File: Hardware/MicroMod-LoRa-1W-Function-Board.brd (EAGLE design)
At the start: 67.5 x 38 mm, 48 parts, among them J11 MICROMOD_STANDARD, Q3 20V/4.2A/52mΩ/1.4W, Q4 600mA/40V, Q5 20V/4.2A/52mΩ/1.4W, Q6 600mA/40V, U1 EEPROM, U4 E19-915M30S

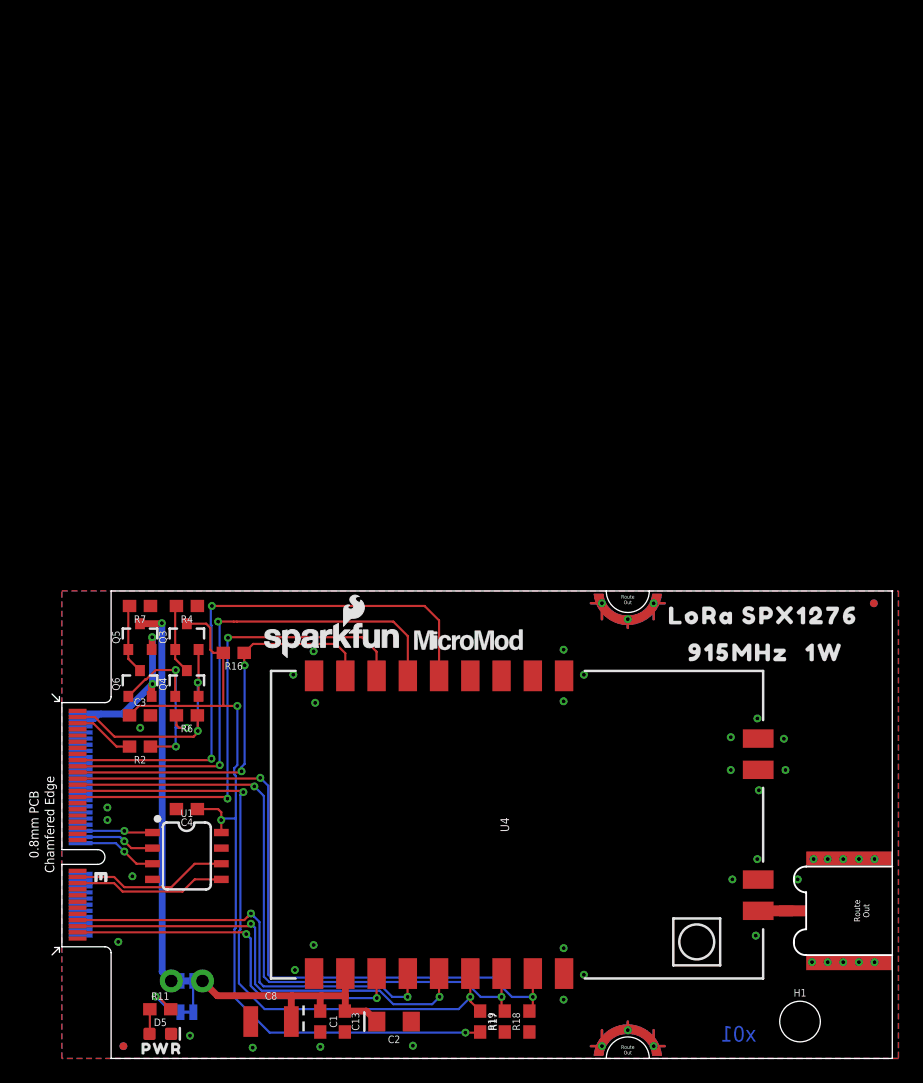
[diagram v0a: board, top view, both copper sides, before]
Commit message: Adding panel files
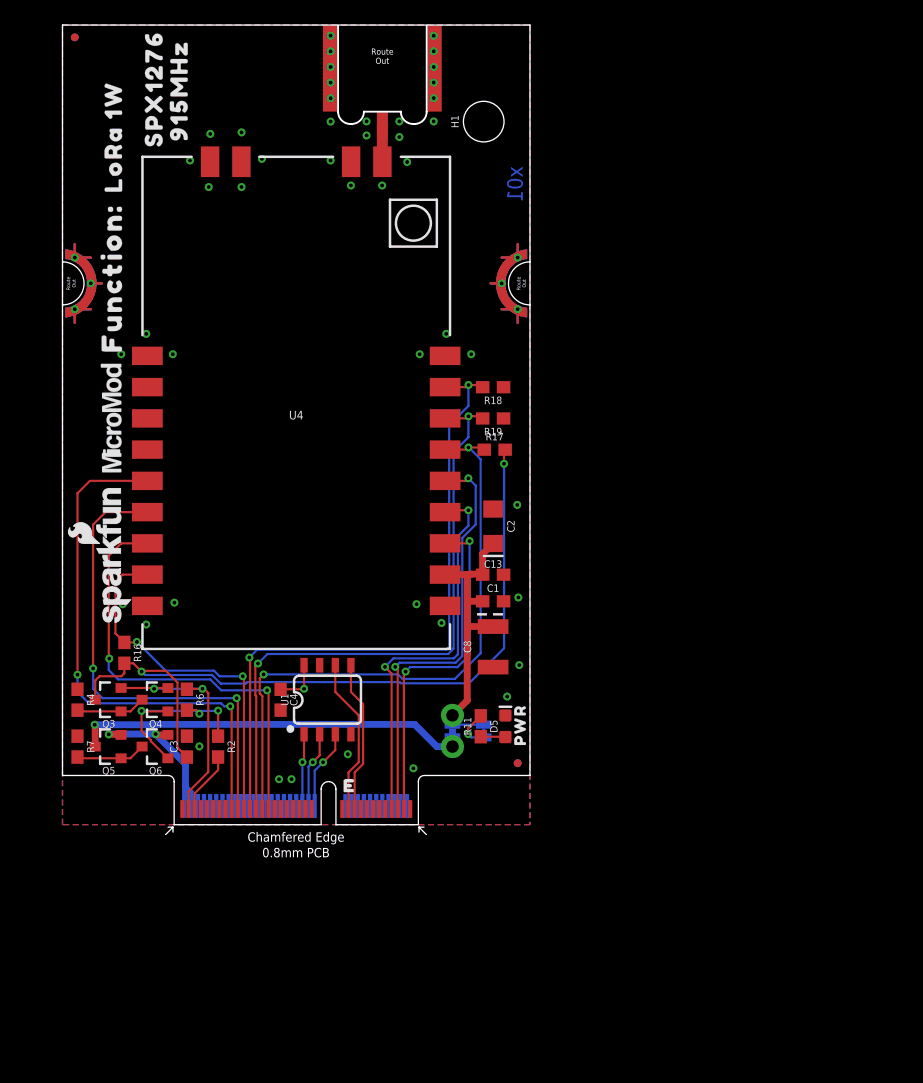
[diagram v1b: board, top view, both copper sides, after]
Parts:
- added LOGO2: SPECIAL_INSTRUCTIONS-ORDERING, SparkFun-Aesthetics:ORDERING_INSTRUCTIONS
- added U$8: (no value), output:FUNCTION#0
- added U$9: (no value), output:#PWR#0
- C8: value 68uF -> 47uF
- J11: device SparkFun-MicroMod-Test:M.2-CARD-E-22_FUNCTION_STANDARD -> SparkFun-MicroMod-Function:M.2-CARD-E-22_FUNCTION_STANDARD
- U$4: device output:#PWR#0 -> output:FUNCTION#0
- moved E1 83.0 mm to (26.1, 65.0), turned to 0 degrees
- moved FD2 79.6 mm to (1.05, 64.0), turned to 90 degrees
- moved FD4 79.6 mm to (1.05, 64.0), turned to 270 degrees
- moved H1 77.5 mm to (34.3, 57.1), turned to 90 degrees
- moved U$2 73.2 mm to (4.19, 58.9), turned to 90 degrees
- moved LOGO3 70.2 mm to (34.3, 52.1), turned to 270 degrees
- moved U$6 67.8 mm to (7.49, 59.8), turned to 90 degrees
- moved U$3 64.5 mm to (9.53, 59.7), turned to 90 degrees
- moved U$5 60.5 mm to (4.19, 54.1), turned to 90 degrees
- moved U$4 52.0 mm to (20.3, 35.6), turned to 270 degrees
- moved R18 51.6 mm to (35.1, 35.6), turned to 180 degrees
- moved R19 49.0 mm to (35.1, 33.0), turned to 180 degrees
- moved R17 46.5 mm to (35.2, 30.5), turned to 0 degrees
- moved C2 41.1 mm to (35.1, 24.3), turned to 270 degrees
- moved U$29 40.4 mm to (22.9, 34.8), turned to 270 degrees
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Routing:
- net LORA_!RST!: track 33.8 -> 29.7 mm
- net LORA_D0: track 39.9 -> 36.1 mm
- net LORA_D2: track 46.9 -> 43.5 mm
- net LORA_D1: track 42.4 -> 39.2 mm
- net LORA_RXEN: track 56.6 -> 54.1 mm
- net SPI_CIPO: track 34.6 -> 32.1 mm
- net SPI_SCK: track 30.8 -> 28.3 mm
- net SPI_COPI: track 37.1 -> 34.6 mm
- net LORA_TXEN: track 53.4 -> 50.9 mm
- net LORA_!CS!: track 52.7 -> 50.3 mm
- net PWR_EN: track 17.8 -> 16.6 mm
- net N$6: track 4.20 -> 3.29 mm
- net GND: vias 40 -> 46
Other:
- board size 67.5 x 38 mm -> 38 x 65 mm
- board text added: "2-Layer"
- board text added: "Beveled Edge"
- board text added: "Board Thickness is 0.8mm"
- board text added: "ENIG Finish"
